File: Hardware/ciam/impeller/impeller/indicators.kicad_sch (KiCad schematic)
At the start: 42 parts, among them J4 Micro-Fit_2x5P, J7 Micro-Fit_2x5P, K1 SRD-05VDC-SL-C, Q5 BSS138

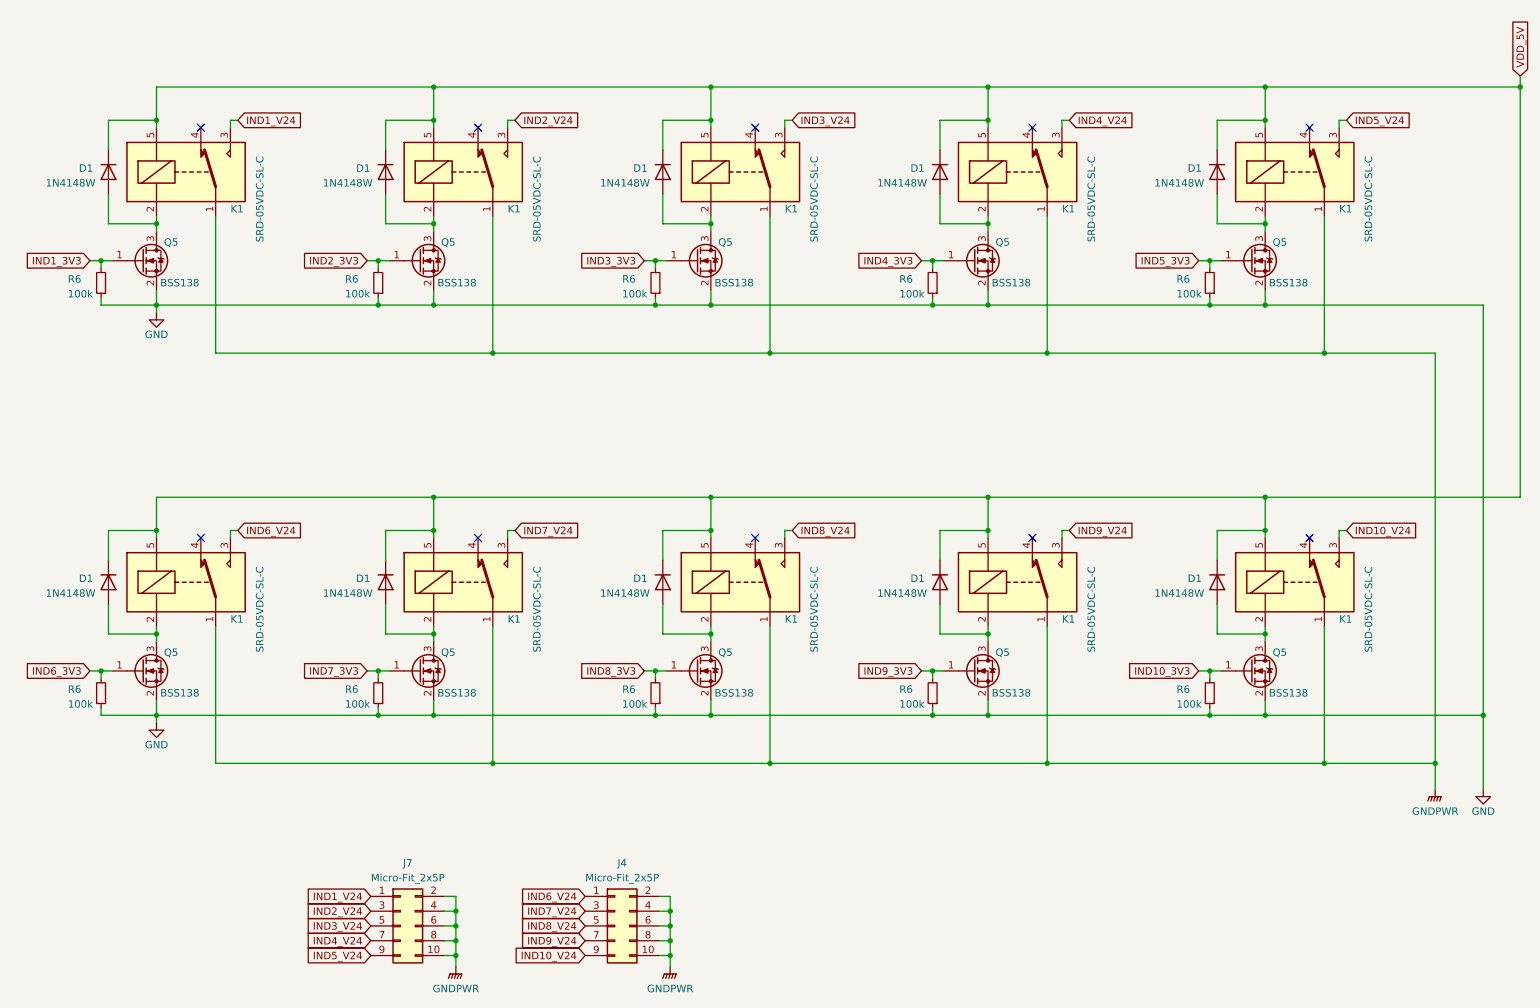
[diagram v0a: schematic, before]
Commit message: updated impeller project
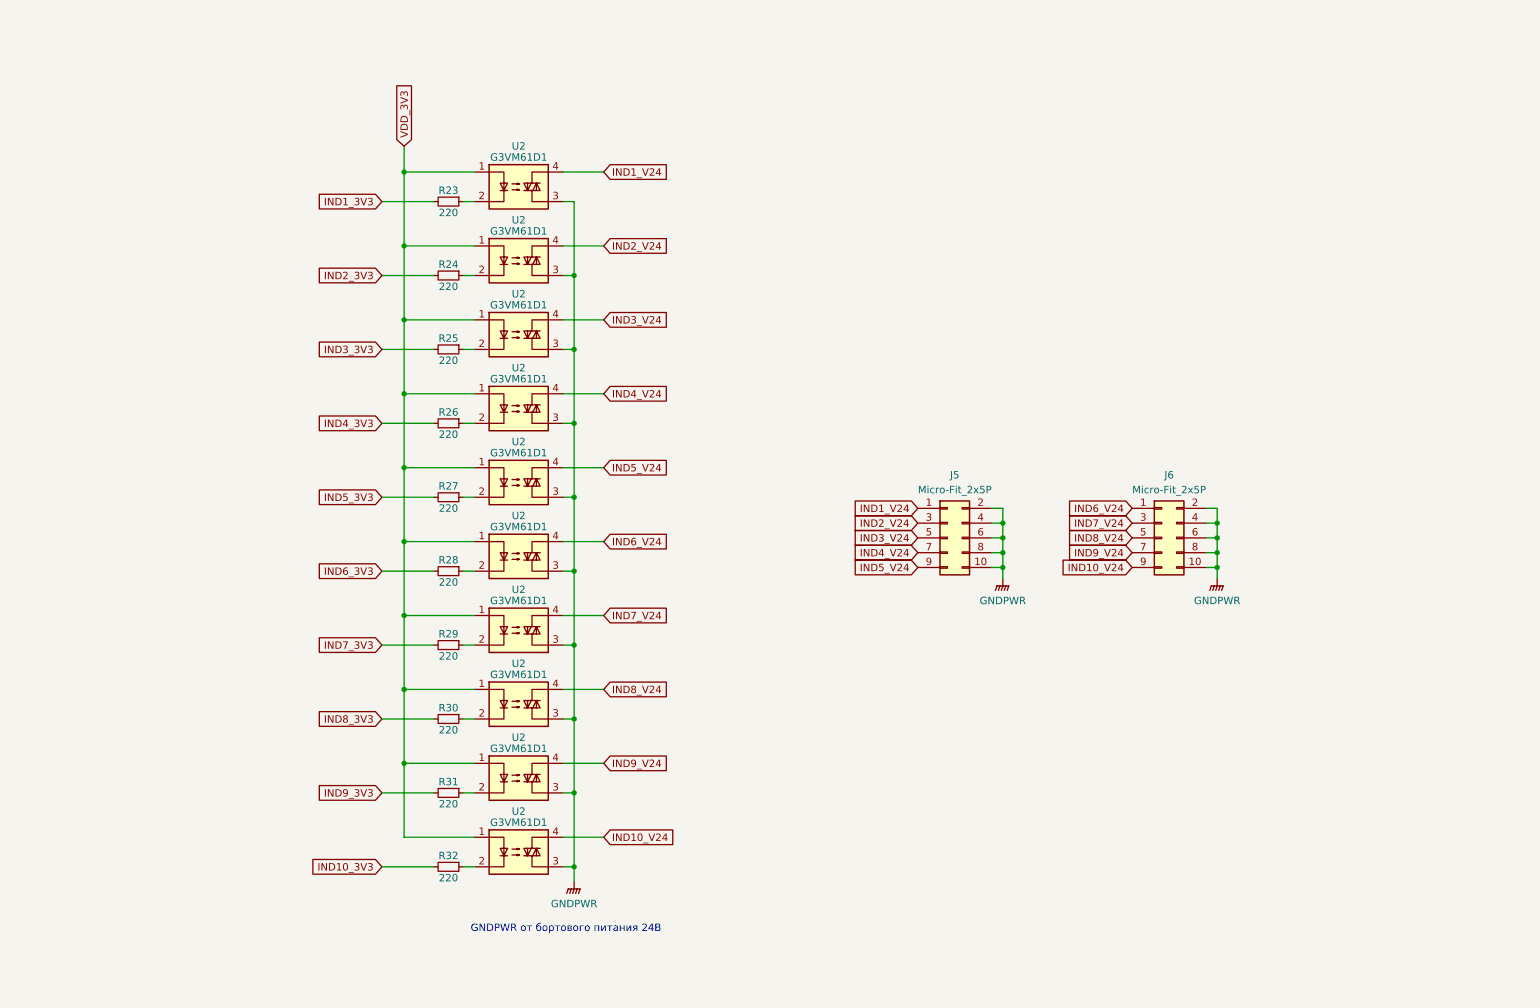
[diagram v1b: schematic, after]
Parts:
- removed D1 (x10): 1N4148W, Diode_SMD:D_SOD-123, symbol Diode:1N4148W
- removed J4, J7: Micro-Fit_2x5P, symbol Connector_Generic:Conn_02x05_Odd_Even
- removed K1 (x10): SRD-05VDC-SL-C, Relay_THT:Relay_SPDT_SANYOU_SRD_Series_Form_C, symbol Relay:SANYOU_SRD_Form_C
- removed Q5 (x10): BSS138, Package_TO_SOT_SMD:SOT-23, symbol Transistor_FET:BSS138
- removed R6 (x10): 100k, Resistor_SMD:R_0603_1608Metric, symbol Device:R_Small
- added J5, J6: Micro-Fit_2x5P, symbol Connector_Generic:Conn_02x05_Odd_Even
- added R23, R24, R25, R26, R27, R28, R29, R30, R31, R32: 220, symbol Device:R_Small
- added U2 (x10): G3VM61D1, symbol Relay_SolidState:S216S01
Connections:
- net GNDPWR: now also J5.10 (Pin_10), J5.2 (Pin_2), J5.4 (Pin_4), J5.6 (Pin_6), J5.8 (Pin_8), J6.10 (Pin_10), J6.2 (Pin_2), J6.4 (Pin_4), J6.6 (Pin_6), J6.8 (Pin_8), U2.3, U2.3, U2.3, U2.3, U2.3, U2.3, U2.3, U2.3, U2.3, U2.3
- net IND10_3V3: now also R32.2
- net IND10_V24: now also J6.9 (Pin_9), U2.4
- net IND1_3V3: now also R23.2
- net IND1_V24: now also J5.1 (Pin_1), U2.4
- net IND2_3V3: now also R24.2
- net IND2_V24: now also J5.3 (Pin_3), U2.4
- net IND3_3V3: now also R25.2
- net IND3_V24: now also J5.5 (Pin_5), U2.4
- net IND4_3V3: now also R26.2
- net IND4_V24: now also J5.7 (Pin_7), U2.4
- net IND5_3V3: now also R27.2
- net IND5_V24: now also J5.9 (Pin_9), U2.4
- net IND6_3V3: now also R28.2
- net IND6_V24: now also J6.1 (Pin_1), U2.4
- net IND7_3V3: now also R29.2
- net IND7_V24: now also J6.3 (Pin_3), U2.4
- net IND8_3V3: now also R30.2
- net IND8_V24: now also J6.5 (Pin_5), U2.4
- net IND9_3V3: now also R31.2
- net IND9_V24: now also J6.7 (Pin_7), U2.4
- new net: R28.1, U2.2
- new net: R24.1, U2.2
- new net: R25.1, U2.2
- new net: R31.1, U2.2
- new net: R32.1, U2.2
- new net: R29.1, U2.2
- new net: R30.1, U2.2
- new net: R27.1, U2.2
- new net: R26.1, U2.2
- new net: R23.1, U2.2
- new net VDD_3V3: U2.1, U2.1, U2.1, U2.1, U2.1, U2.1, U2.1, U2.1, U2.1, U2.1
- no-connect marks 10 -> 0
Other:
- note added: "GNDPWR от бортового питания 24В"
